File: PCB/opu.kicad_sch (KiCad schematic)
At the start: 1 part, among them J2 Conn_02x12_Odd_Even

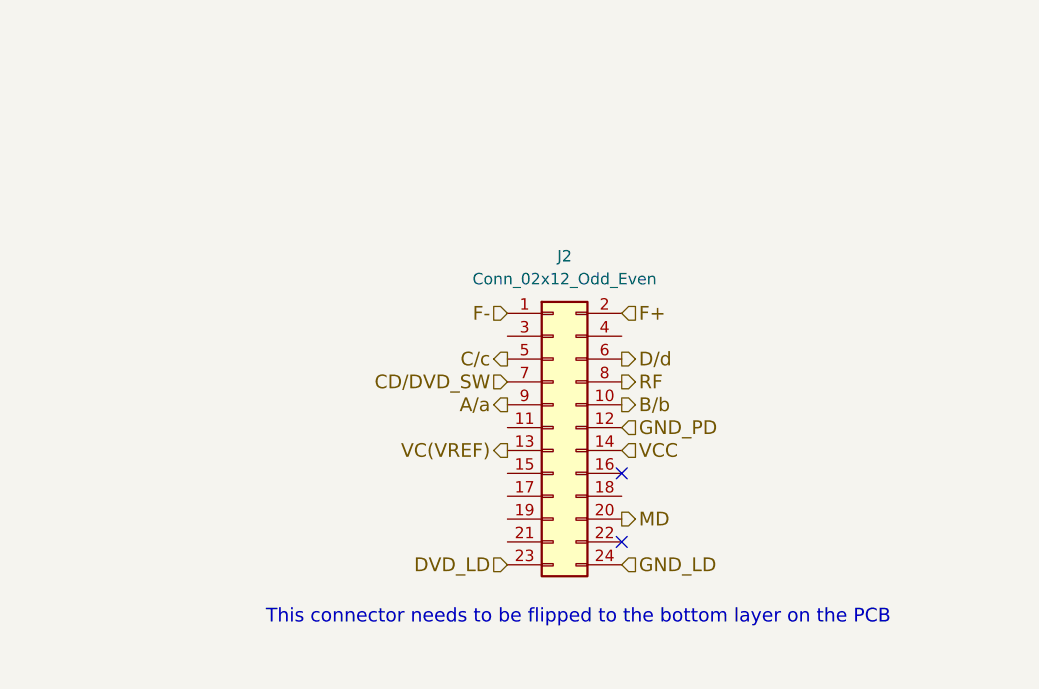
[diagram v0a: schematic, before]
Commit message: Modify PCB
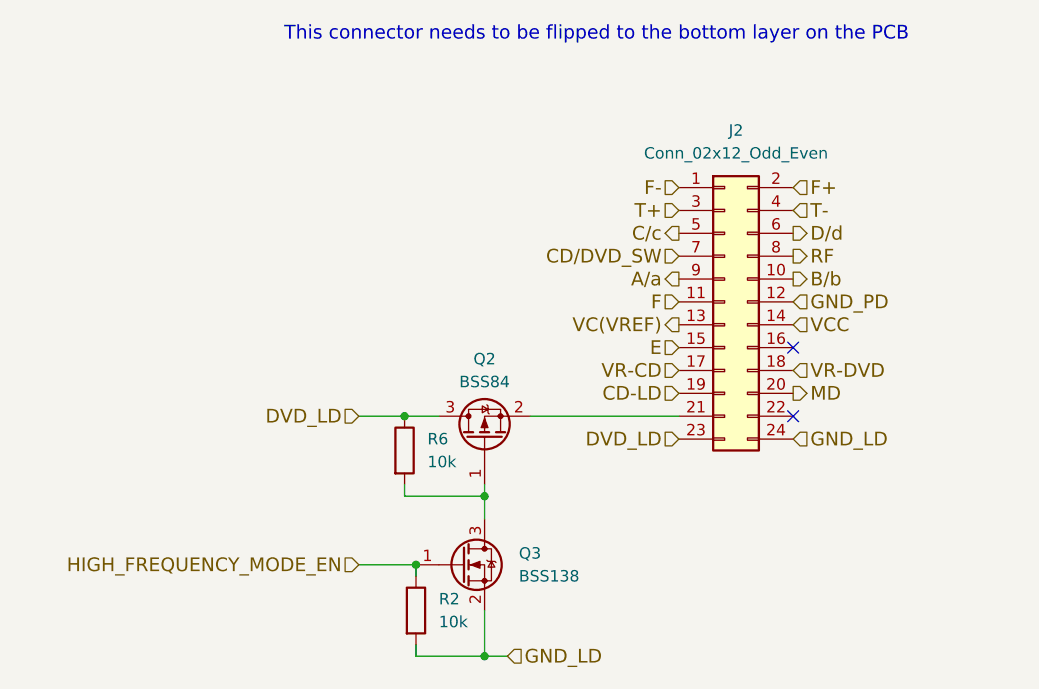
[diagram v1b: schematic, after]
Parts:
- added Q2: BSS84, Package_TO_SOT_SMD:SOT-23, symbol Transistor_FET:BSS84
- added Q3: BSS138, Package_TO_SOT_SMD:SOT-23, symbol Transistor_FET:BSS138
- added R2, R6: 10k, symbol Device:R
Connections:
- net DVD_LD: now also Q2.3 (D), R6.1
- net GND_LD: now also Q3.2 (S), R2.2
- net F: now reaches J2.11 (Pin_11)
- net E: now reaches J2.15 (Pin_15)
- net VR-CD: now reaches J2.17 (Pin_17)
- net VR-DVD: now reaches J2.18 (Pin_18)
- net CD-LD: now reaches J2.19 (Pin_19)
- net at J2.21 (Pin_21): now also Q2.2 (S)
- net T+: now reaches J2.3 (Pin_3)
- net T-: now reaches J2.4 (Pin_4)
- new net: Q2.1 (G), Q3.3 (D), R6.2
- new net HIGH_FREQUENCY_MODE_EN: Q3.1 (G), R2.1
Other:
- moved on the sheet: J2
